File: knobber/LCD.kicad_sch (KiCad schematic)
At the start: 1 part, among them J901 Conn_01x08_Socket

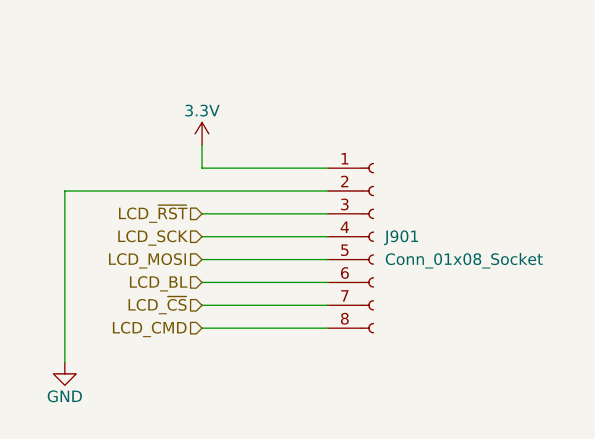
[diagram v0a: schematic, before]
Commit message: Updated schematic & PCB
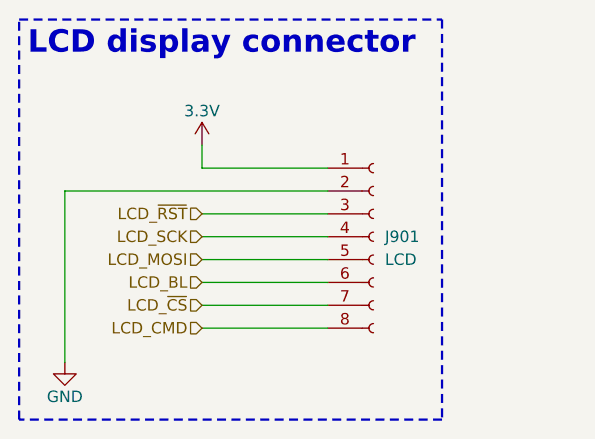
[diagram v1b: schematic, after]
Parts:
- J901: value Conn_01x08_Socket -> LCD
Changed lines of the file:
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@@
 	(title_block
 		(title "LCD")
-		(date "2026-03-14")
+		(date "2026-03-16")
 		(rev "V0.1")
 		(company "Author: Emiel V")
+	)
+	(text_box "LCD display connector"
+		(exclude_from_sim no)
+		(at 85.09 43.18 0)
+		(size 46.99 44.45)
+		(margins 0.9525 0.9525 0.9525 0.9525)
+		(stroke
+			(width 0.25)
+			(type dash)
+		)
+		(fill
+			(type none)
+		)
+		(effects
+			(font
+				(size 2.5 2.5)
+				(thickness 0.5)
+				(bold yes)
+			)
+			(justify left top)
+		)
 	)
 	(wire
@@
 			)
 		)
-		(property "Value" "Conn_01x08_Socket"
+		(property "Value" "LCD"
 			(at 125.73 69.8499 0)
 			(effects
